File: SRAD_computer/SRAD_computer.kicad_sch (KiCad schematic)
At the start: 66 parts, among them J1 Terminal_3, J2 Conn_01x02, J3 UJ20-C-H-G-SMT-1-P16-TR, J4 Terminal_2, J5 Connector_3_Pol, J6 Micro_SD_Card, Q1 MMBT5551L, Q3 FDN340P, U1 NCP1117-3.3_SOT223, U2 W25Q128JVS, U3 RP2040, U4 BME280, U5 MPU-9250, U6 SAM-M8Q-0-10, Y1 Crystal

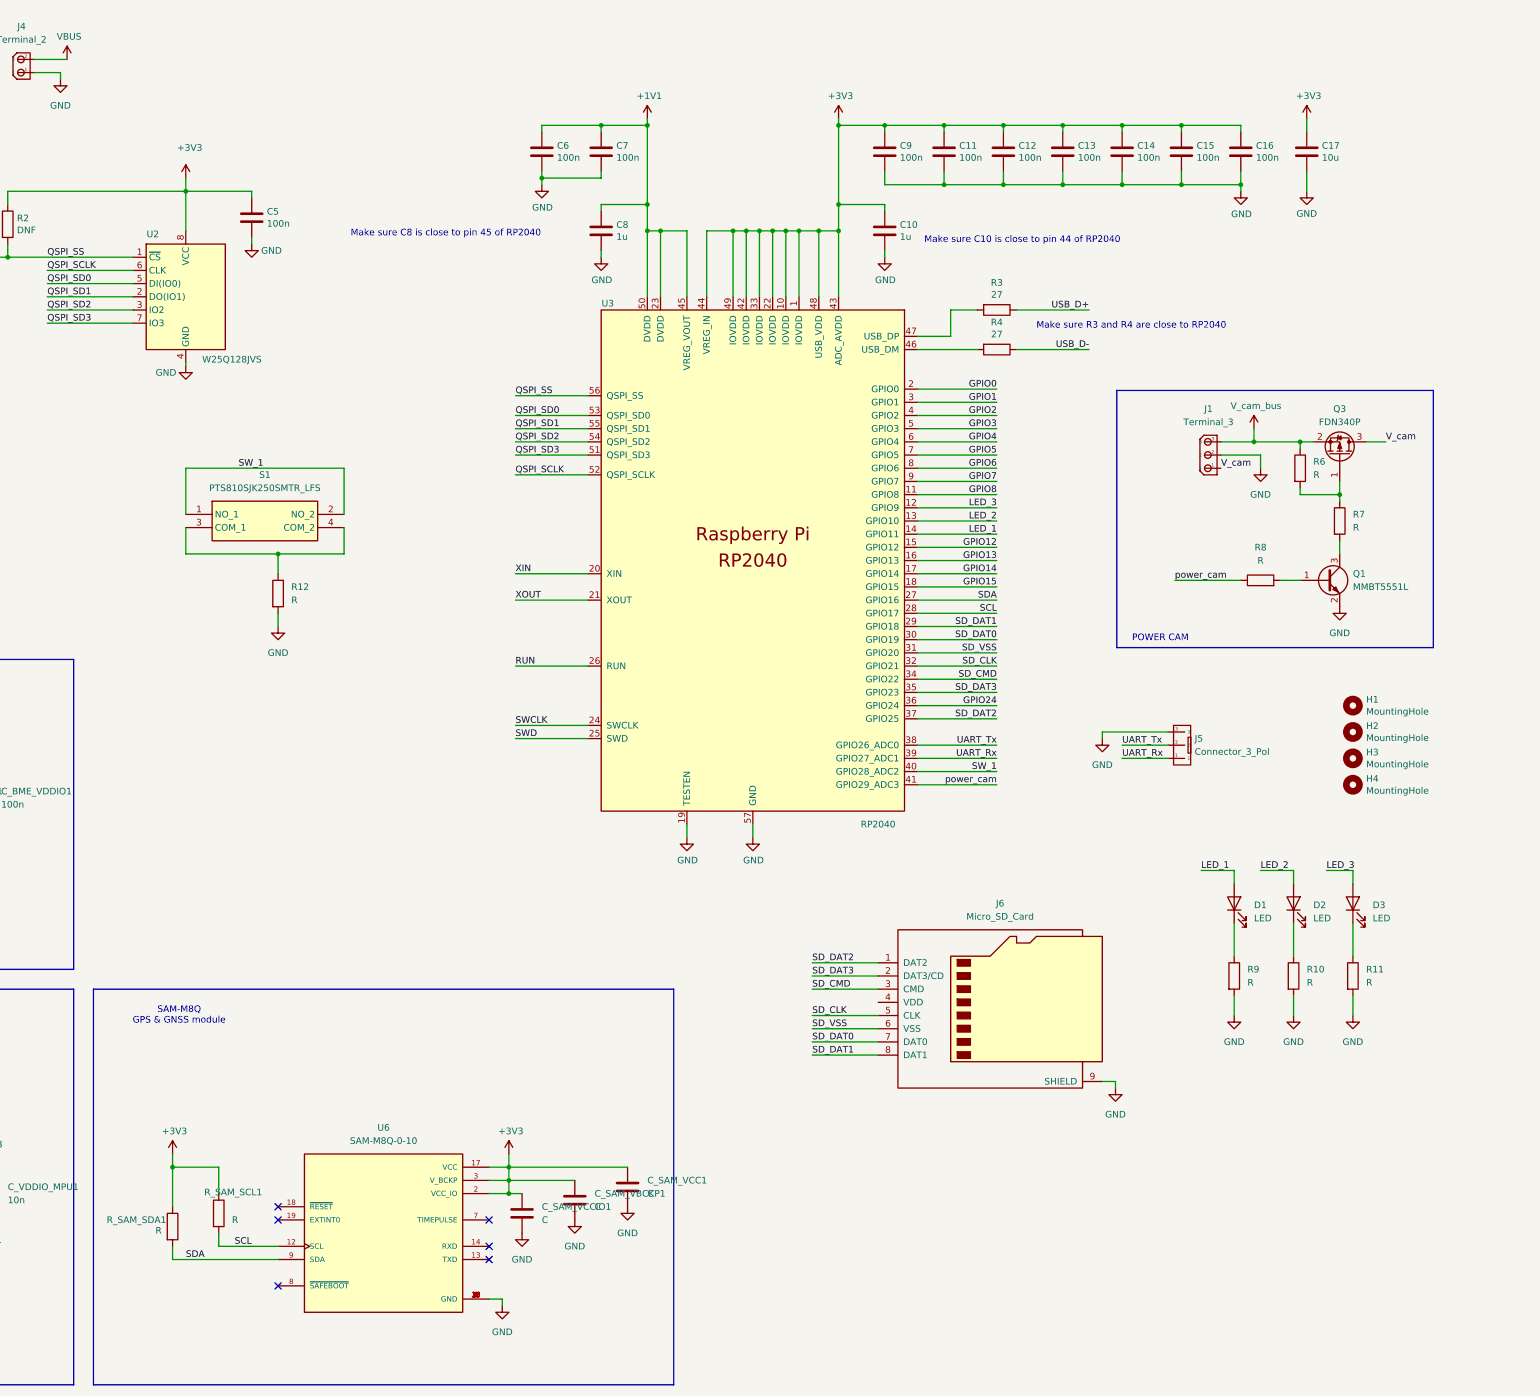
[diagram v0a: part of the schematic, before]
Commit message: SD layout
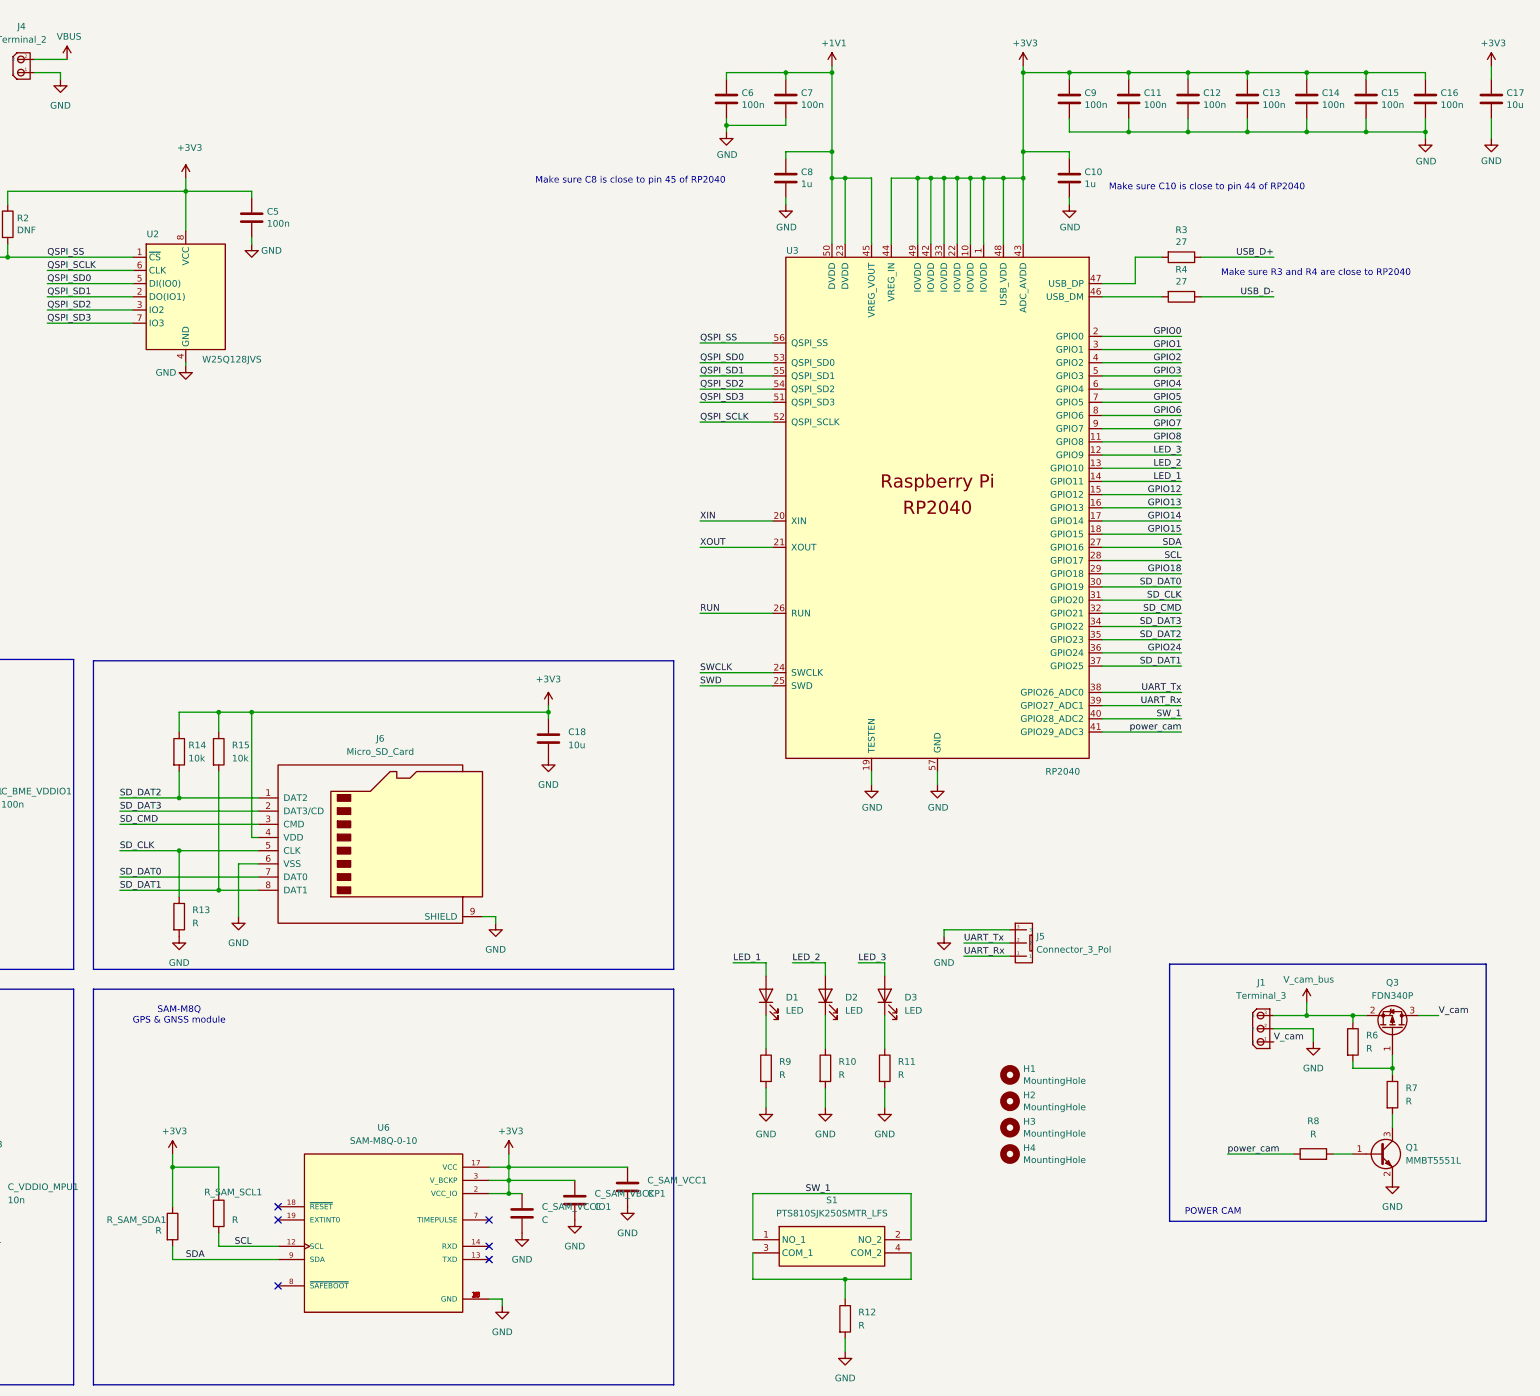
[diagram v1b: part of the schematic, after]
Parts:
- added C18: 10u, TCLib:C_0805, symbol TCLib:C
- added R13: R, TCLib:R_0805, symbol TCLib:R
- added R14, R15: 10k, TCLib:R_0805, symbol TCLib:R
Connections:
- net +3V3: now also J6.4 (VDD), C18.1, R14.1, R15.1
- net GND: now also J6.6 (VSS), C18.2, R13.2
- net SD_CLK: now also U3.31 (GPIO20), R13.1; no longer U3.32 (GPIO21)
- net SD_CMD: now also U3.32 (GPIO21); no longer U3.34 (GPIO22)
- net SD_DAT1: now also U3.37 (GPIO25), R15.2; no longer U3.29 (GPIO18)
- net SD_DAT2: now also U3.35 (GPIO23), R14.2; no longer U3.37 (GPIO25)
- net SD_DAT3: now also U3.34 (GPIO22); no longer U3.35 (GPIO23)
- removed net SD_VSS: J6.6 (VSS), U3.31 (GPIO20)
- new net GPIO18: U3.29 (GPIO18)
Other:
- moved on the sheet: C10, C11, C12, C13, C14, C15, C16, C17, C6, C7, C8, C9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
